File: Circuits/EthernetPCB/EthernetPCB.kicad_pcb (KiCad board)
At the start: 2 copper layers, 41 x 26 mm, 3 parts, among them J1 Conn_02x03_Counter_Clockwise

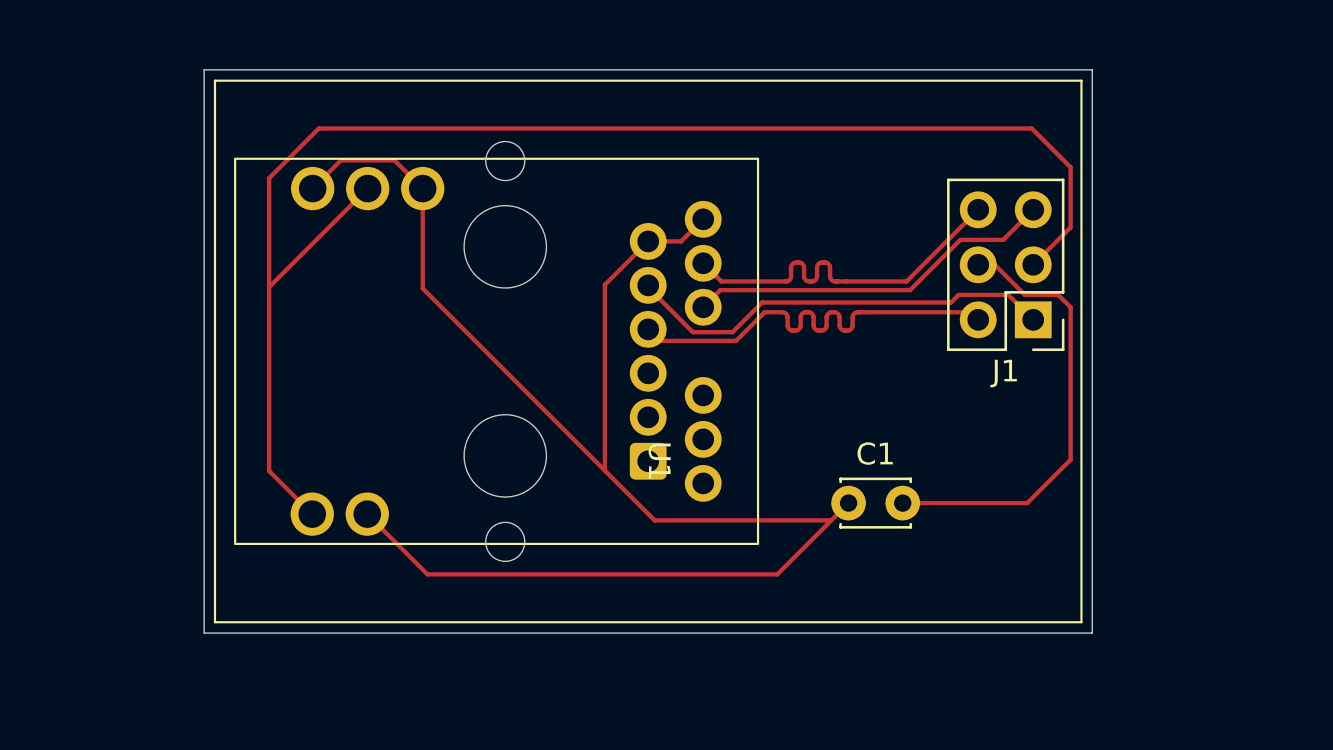
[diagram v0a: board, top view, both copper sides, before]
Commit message: Final output in thermocouple and ethernet pcb
Verified. Ground plane added. All systems normal.
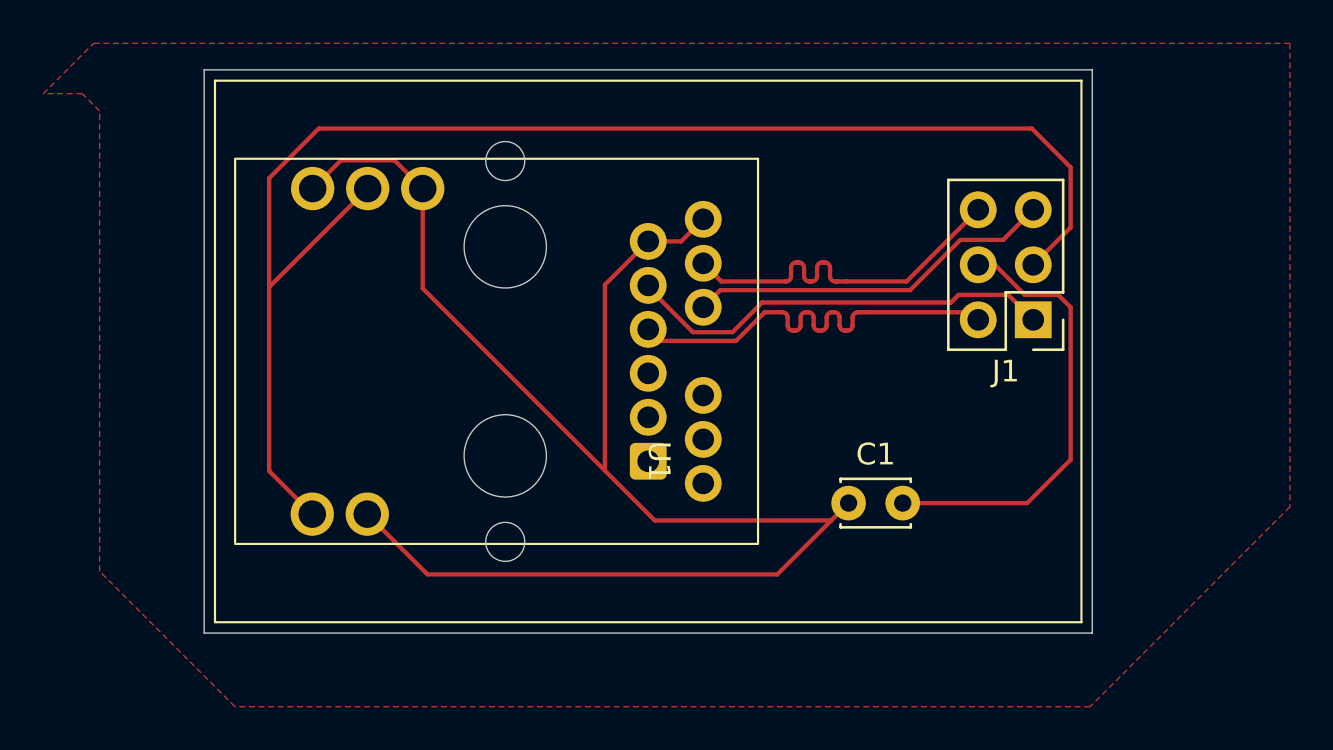
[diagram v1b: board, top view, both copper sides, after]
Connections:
- net Net-(J1-Pin_4) renamed GND
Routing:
- added copper zone on F.Cu, net GND
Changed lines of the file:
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@@
 	(net 10 "unconnected-(U1-MDCT4-Pad7)")
 	(net 11 "unconnected-(U1-MD3+-Pad3)")
-	(net 12 "Net-(J1-Pin_4)")
+	(net 12 "GND")
 	(net 13 "Net-(J1-Pin_3)")
 	(footprint "EthernetPCB:LINK-PP LPJK7003B97NL"
@@
 			(layers "*.Cu" "*.Mask")
 			(remove_unused_layers no)
-			(net 12 "Net-(J1-Pin_4)")
+			(net 12 "GND")
 			(pinfunction "Pin_4")
 			(pintype "passive")
@@
 			(layers "*.Cu" "*.Mask")
 			(remove_unused_layers no)
-			(net 12 "Net-(J1-Pin_4)")
+			(net 12 "GND")
 			(pintype "passive")
 		)
@@
 		(net 13)
 	)
+	(zone
+		(net 12)
+		(net_name "GND")
+		(layer "F.Cu")
+		(hatch edge 0.5)
+		(connect_pads
+			(clearance 0.5)
+		)
+		(min_thickness 0.25)
+		(filled_areas_thickness no)
+		(fill yes
+			(thermal_gap 0.5)
+			(thermal_bridge_width 0.5)
+			(island_removal_mode 2)
+			(island_area_min 10)
+		)
+		(polygon
+			(pts
+				(xy 168.125 80.275) (xy 168.125 101.675) (xy 158.9 110.9) (xy 119.425 110.9) (xy 113.175 104.65)
+				(xy 113.175 83.4) (xy 112.375 82.6) (xy 110.575 82.6) (xy 112.9 80.275)
+			)
+		)
+	)
 	(generated
